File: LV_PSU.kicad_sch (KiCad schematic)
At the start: 26 parts, among them IC201 1769205241, J201 Header_Male_Pin_2.54mm_1X2_,_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, J202 PJ-082BH, U201 OKI-78SR-5_1.5-W36H-C, U202 AZ1117IH-3.3TRG1, U203 AZ1117IH-3.3TRG1

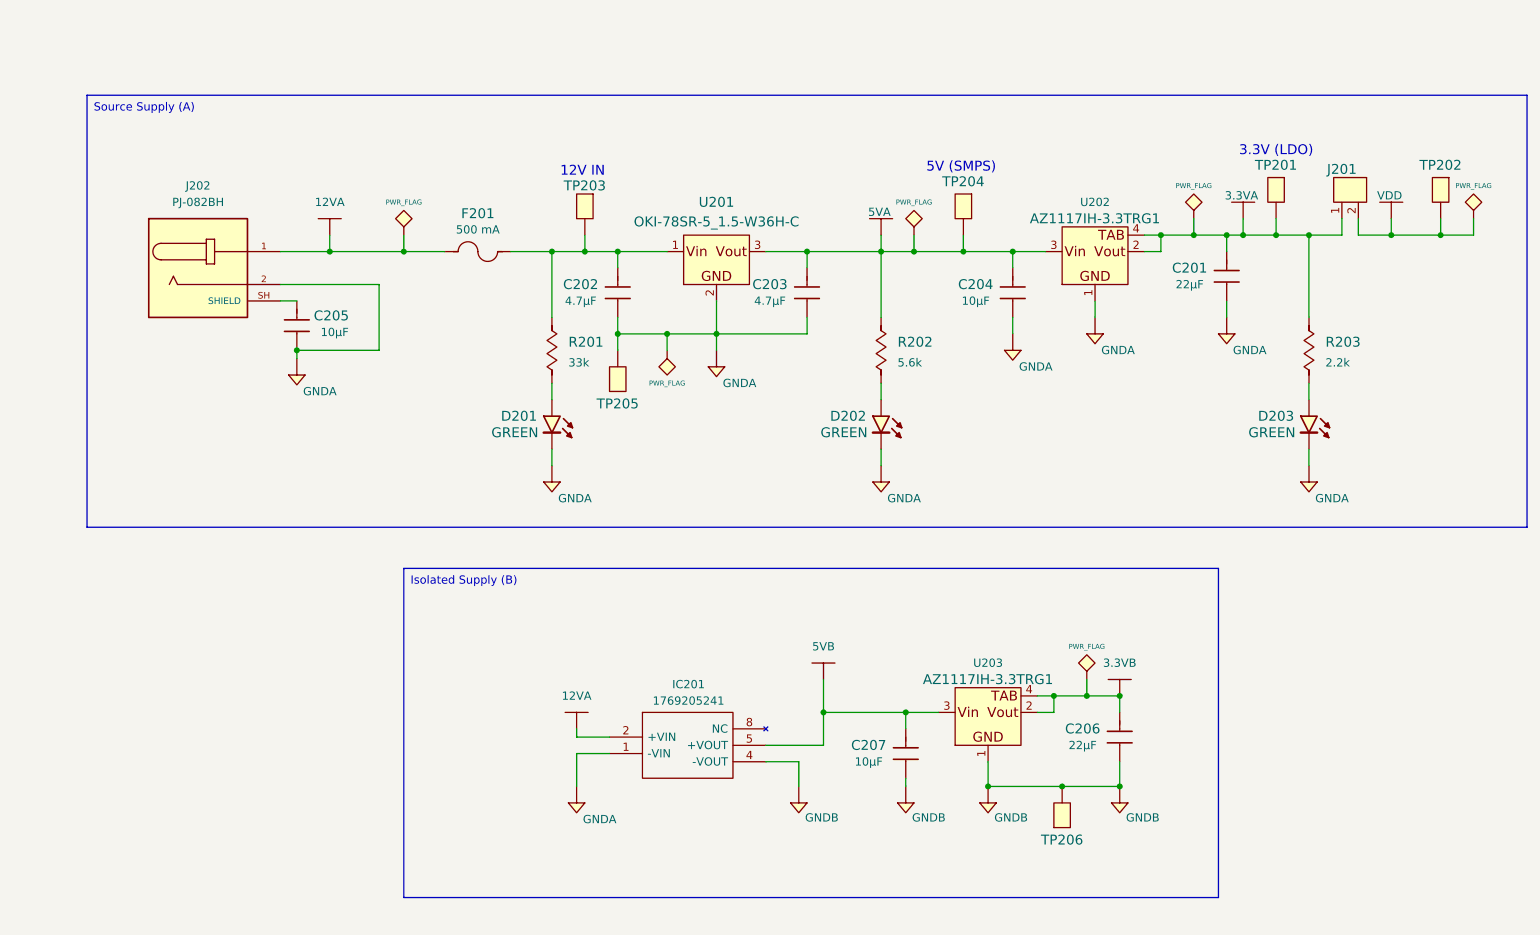
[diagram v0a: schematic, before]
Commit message: modif schématique
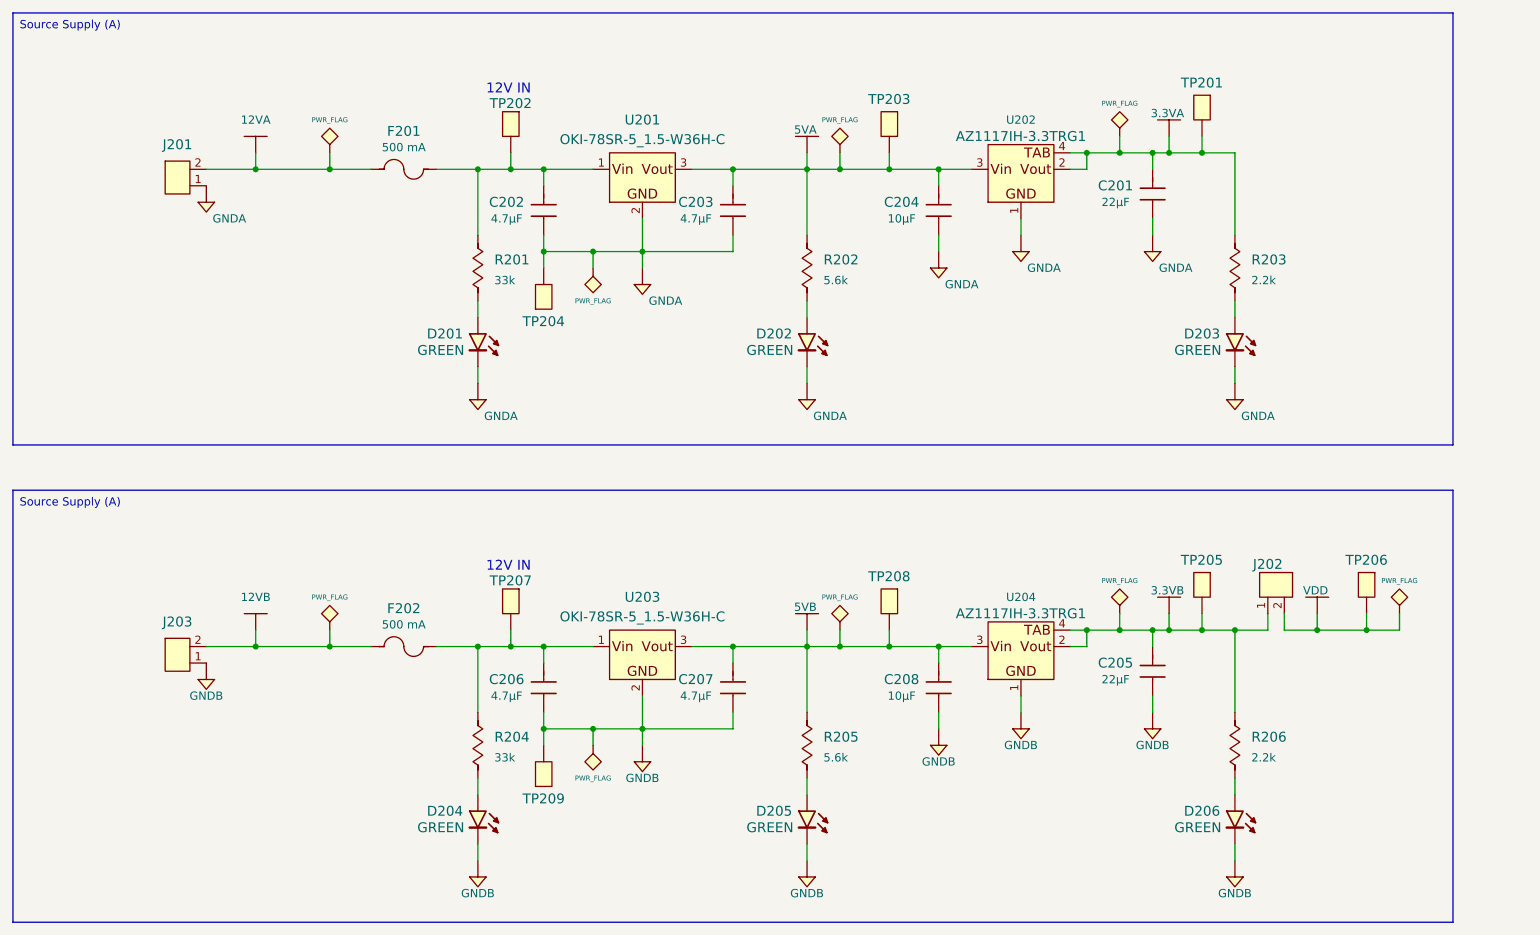
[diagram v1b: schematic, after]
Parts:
- removed C205, C207: 885012107014, Capacitors:C0805, symbol Capacitors:885012107014
- removed C206: 885012107005, Capacitors:C0805, symbol Capacitors:885012107005
- removed IC201: 1769205241, IC:1769205241, symbol PMIC:1769205241
- removed J201: Header_Male_Pin_2.54mm_1X2_,_Unshrouded, Connectors:Headers_2.54mm_1X2, symbol Connectors:Header_Male_Pin_2.54mm_1X2_,_Unshrouded
- removed J202: PJ-082BH, Connectors:CUI_PJ-082BH, symbol Connectors:PJ-082BH
- removed TP202: Test_Point_THM, Connectors:Keystone_5001, symbol Connectors:Test_Point_THM
- removed U203: AZ1117IH-3.3TRG1, IC:SOT-223-3, symbol PMIC:AZ1117IH-3.3TRG1
- added C205: 885012107005, Capacitors:C0805, symbol Capacitors:885012107005
- added C206, C207: 885012107018, Capacitors:C0805, symbol Capacitors:885012107018
- added C208: 885012107014, Capacitors:C0805, symbol Capacitors:885012107014
- added D204, D205, D206: 150080VS75000, Diodes:LED_0805_GREEN, symbol Diodes:150080VS75000
- added F202: 39511000440, Fuses:TE5_395, symbol Fuses:39511000440
- added J201, J203: 1935161, Connectors:1935161, symbol Connectors:1935161
- added J202: Header_Male_Pin_2.54mm_1X2_,_Unshrouded, Connectors:Headers_2.54mm_1X2, symbol Connectors:Header_Male_Pin_2.54mm_1X2_,_Unshrouded
- added R204: RC0805JR-0733KL, Resistors:R0805, symbol Resistors:RC0805JR-0733KL
- added R205: RC0805FR-075K6L, Resistors:R0805, symbol Resistors:RC0805FR-075K6L
- added R206: RC0805JR-072K2L, Resistors:R0805, symbol Resistors:RC0805JR-072K2L
- added TP205, TP207, TP208, TP209: Test_Point_THM, Connectors:Keystone_5001, symbol Connectors:Test_Point_THM
- added U203: OKI-78SR-5_1.5-W36H-C, Assembly:OKI-78SR_Horizontal, symbol PMIC:OKI-78SR-5_1.5-W36H-C
- added U204: AZ1117IH-3.3TRG1, IC:SOT-223-3, symbol PMIC:AZ1117IH-3.3TRG1
- renumbered TP203 to TP202, TP204 to TP203, TP205 to TP204
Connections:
- net 12VA: now also J201.2
- net 3.3VB: now also C205.2, J202.1, R206.2, TP205.1 (TP), U204.2 (Vout), U204.4 (Vout_(TAB))
- net 5VB: now also C207.2, C208.2, R205.2, TP208.1 (TP), U203.3 (Vout), U204.3 (Vin)
- net GNDA: now also J201.1
- net GNDB: now also C205.1, C206.1, C207.1, C208.1, D204.1 (Cathode), D205.1 (Cathode), D206.1 (Cathode), J203.1, TP209.1 (TP), U203.2 (GND), U204.1 (GND); no longer TP206.1 (TP)
- net VDD: now also TP206.1 (TP), J202.2
- new net: D205.2 (Anode), R205.1
- new net: C206.2, F202.2, R204.2, TP207.1 (TP), U203.1 (Vin)
- new net: D206.2 (Anode), R206.1
- new net: D204.2 (Anode), R204.1
- new net 12VB: F202.1, J203.2
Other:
- note removed: "3.3V (LDO)"
- note removed: "5V (SMPS)"
- moved on the sheet: C201, C202, C203, C204, D201, D202, D203, F201, R201, R202, R203, TP201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
